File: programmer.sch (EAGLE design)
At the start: 15 parts, among them U1 ATMEGA8U2AU, X1 16MHz

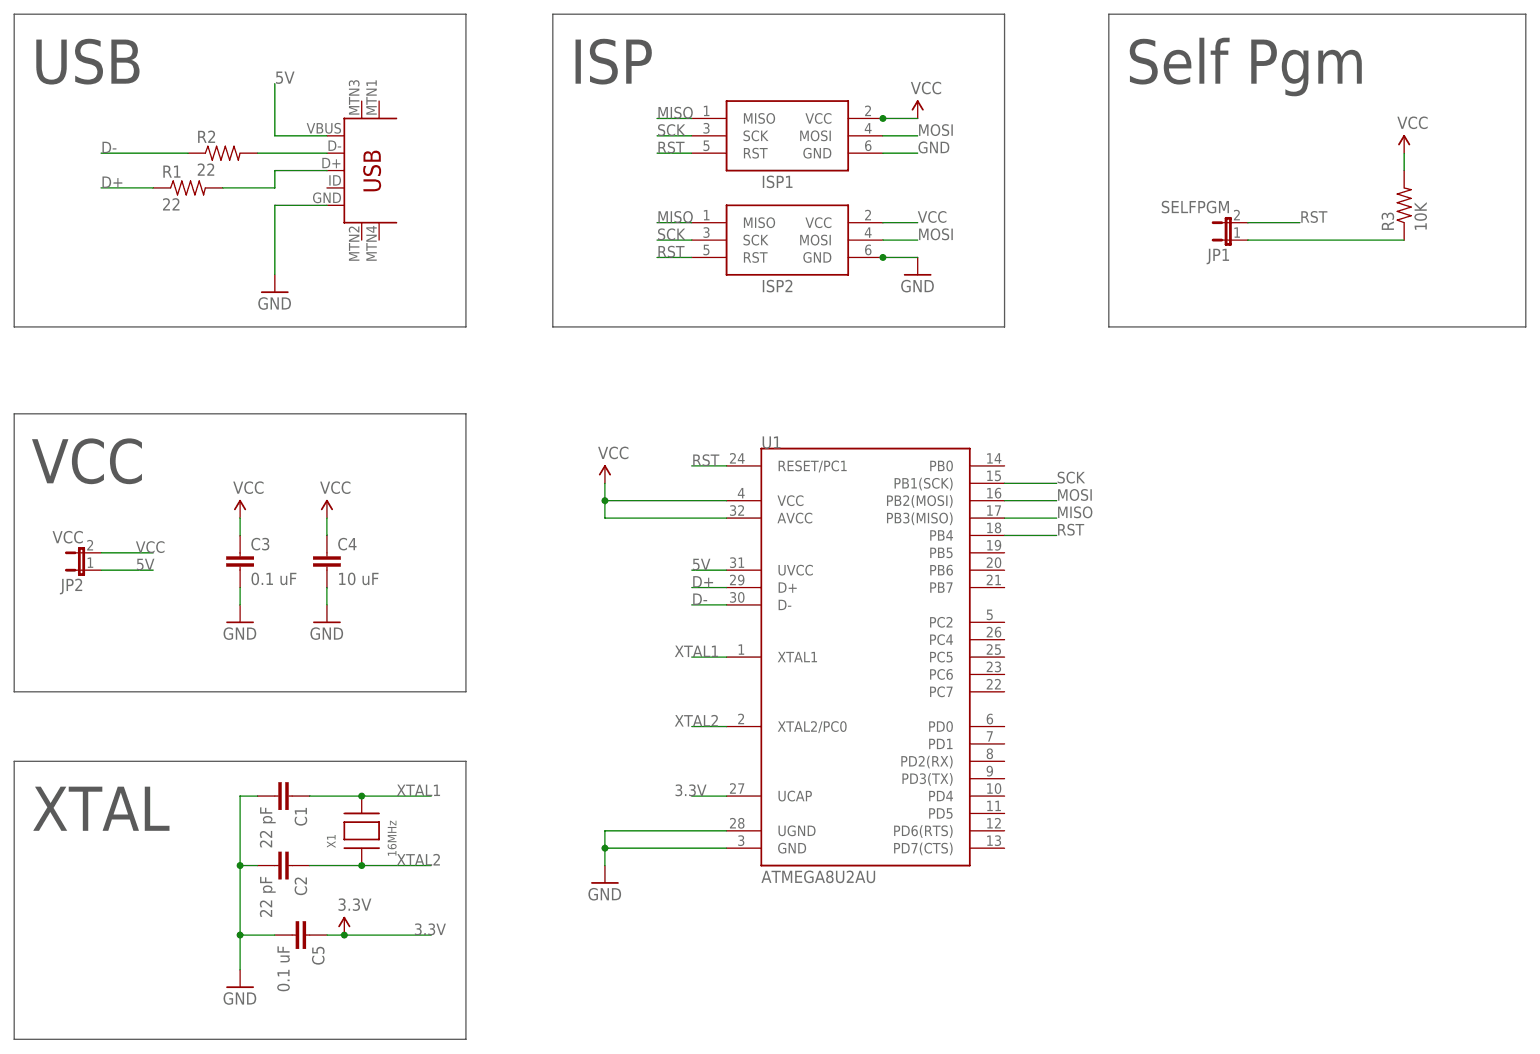
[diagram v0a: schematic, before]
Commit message: Blinkenlights.
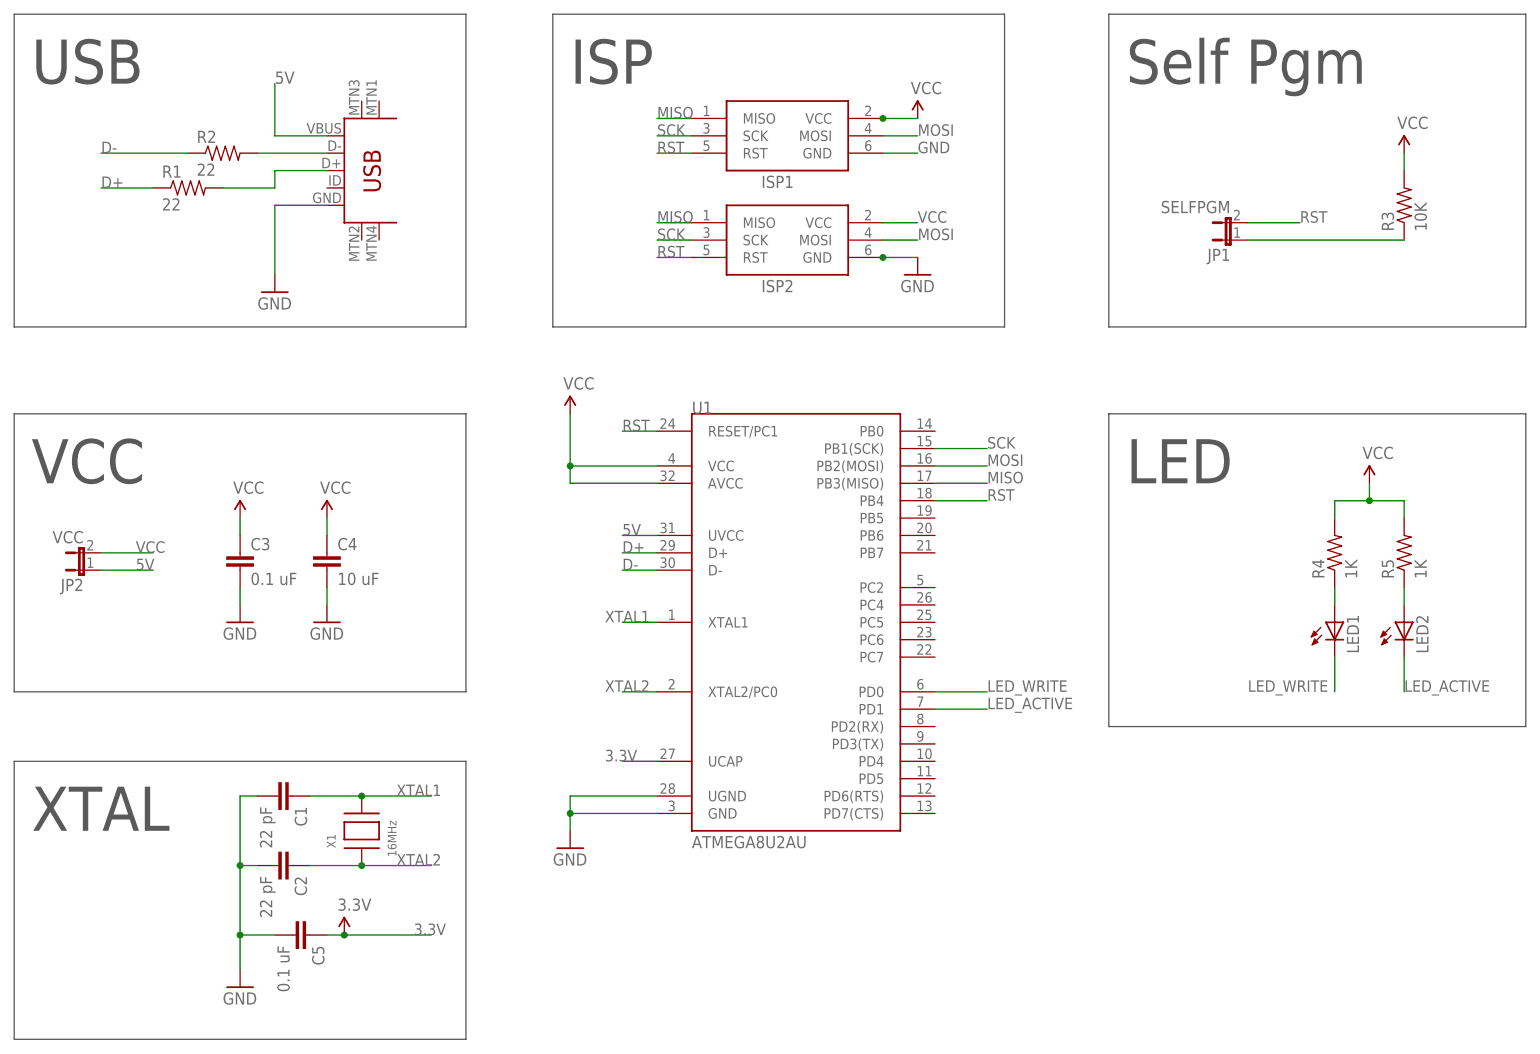
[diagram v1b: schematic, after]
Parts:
- added LED1, LED2: (no value), adafruit:LEDSMT1206
- added R4, R5: 1K, SparkFun:RESISTOR0805-RES
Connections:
- new net LED_ACTIVE: LED2.C, U1.PD1
- new net LED_WRITE: LED1.C, U1.PD0
- new net N$1: LED2.A, R5.1
- new net N$3: LED1.A, R4.1
- net VCC: now also R4.2, R5.2
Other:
- note added: "LED"
- moved on the sheet: U1
